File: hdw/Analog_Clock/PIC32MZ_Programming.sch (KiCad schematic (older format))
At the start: 10 parts

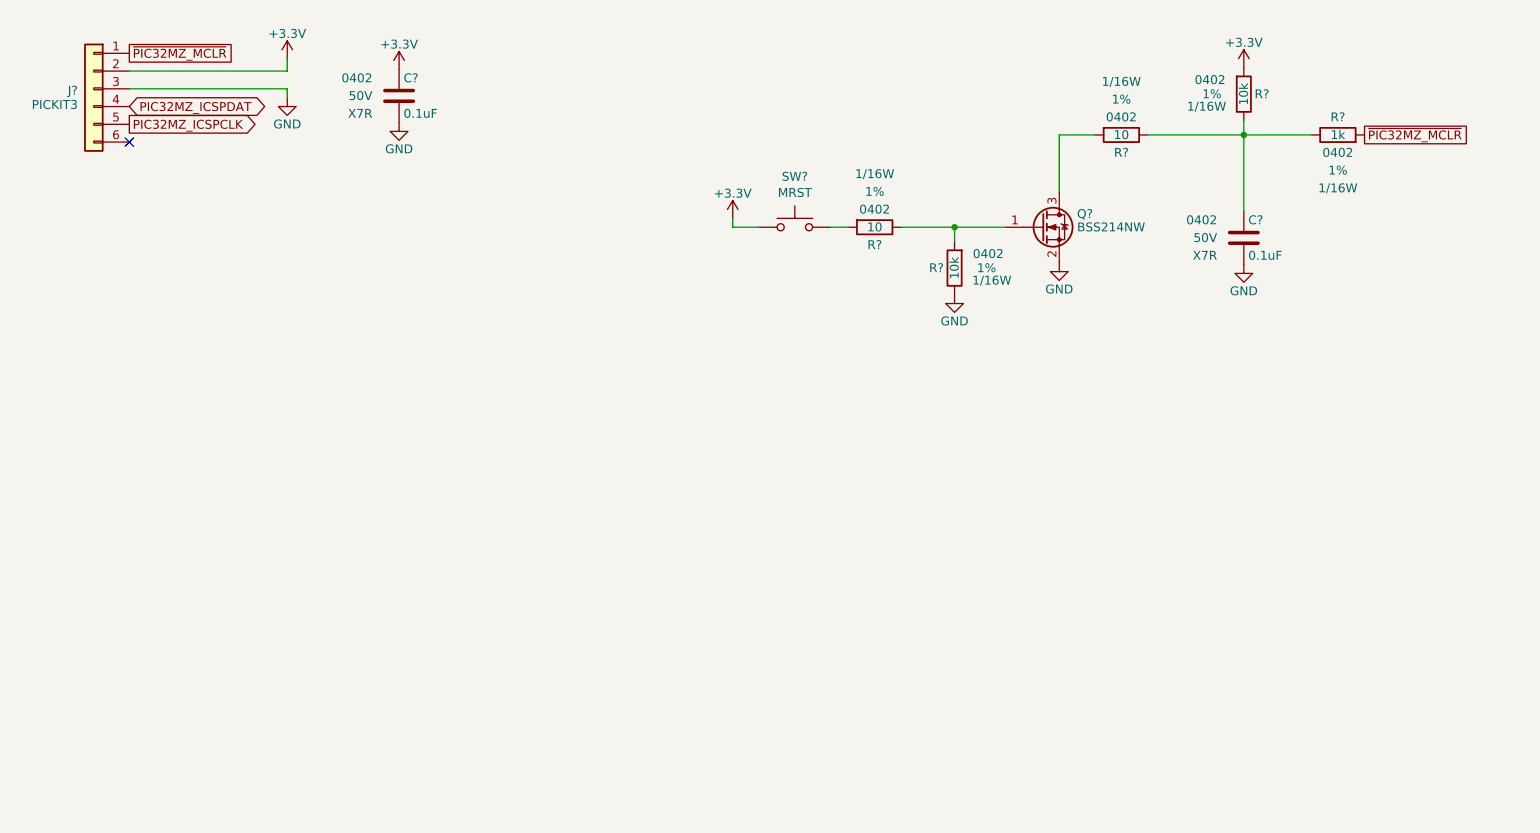
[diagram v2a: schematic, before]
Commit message: more analog work, added some more sch stuff
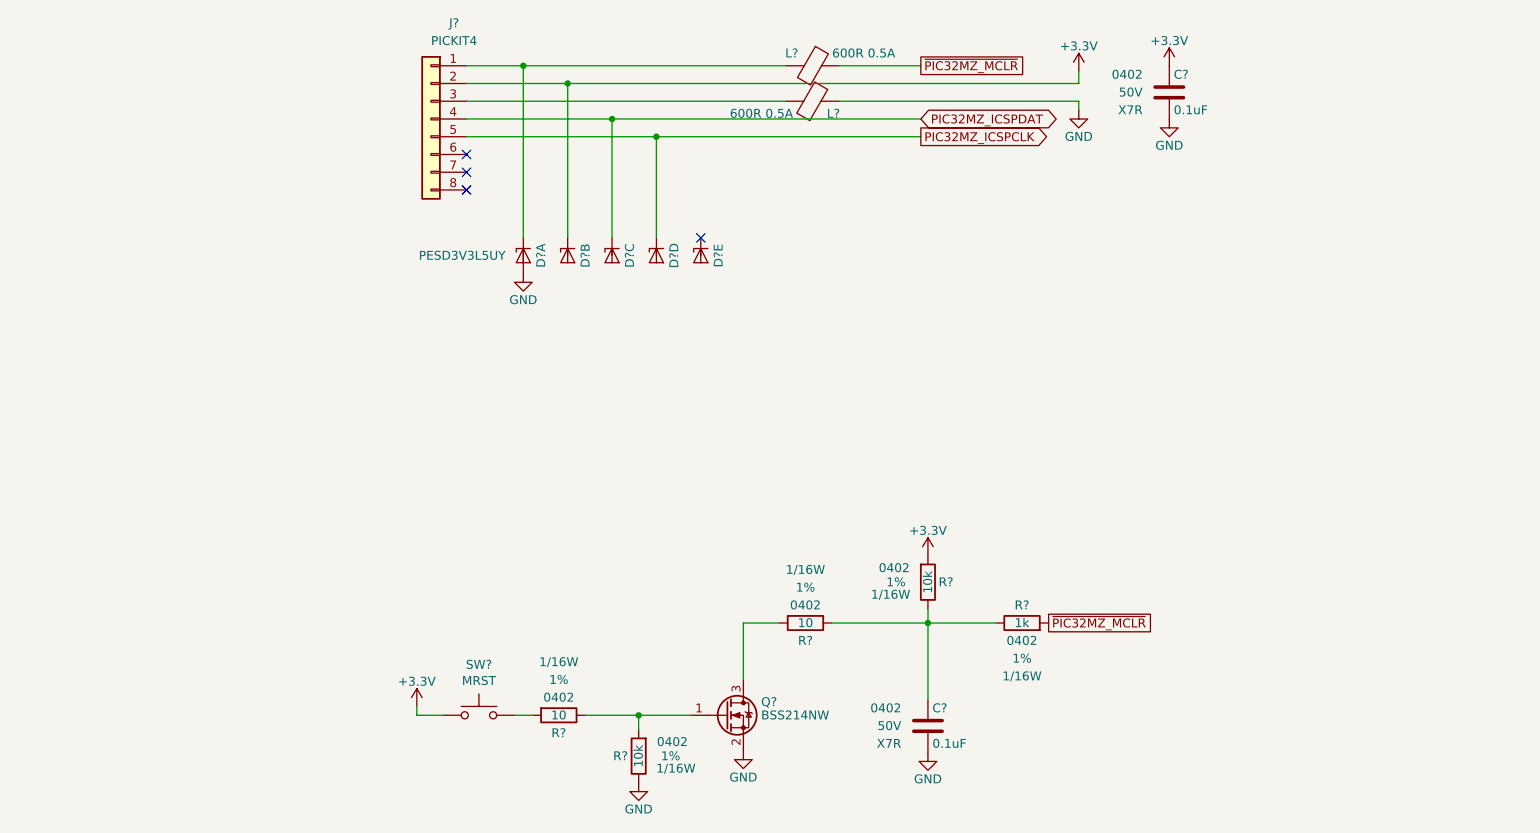
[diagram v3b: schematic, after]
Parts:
- removed J?: PICKIT3, Custom Footprints Library:PICKIT3_Header, symbol Connector_Generic:Conn_01x06
- added D? (x5): PESD3V3L5UY, Package_TO_SOT_SMD:SOT-363_SC-70-6, symbol Power_Protection:PESD3V3L5UY
- added J?: PICKIT4, Custom Footprints Library:PICKIT4_Header, symbol Connector_Generic:Conn_01x08
- added L? (x2): 600R 0.5A, Inductors_SMD:L_0402, symbol Device:Ferrite_Bead
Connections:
- net +3V3: now also D?.3 (K2), J?.2 (Pin_2)
- net GND: now also D?.2 (A), L?.2
- net PIC32MZ_ICSPCLK: now also D?.5 (K4), J?.5 (Pin_5)
- net PIC32MZ_ICSPDAT: now also D?.4 (K3), J?.4 (Pin_4)
- net ~PIC32MZ_MCLR: now also L?.1
- new net: D?.1 (K1), J?.1 (Pin_1), L?.2
- new net: J?.3 (Pin_3), L?.1
- no-connect marks 1 -> 4
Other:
- moved on the sheet: C?, Q?, R?, SW?
